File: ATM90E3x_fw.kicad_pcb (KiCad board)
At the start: 2 copper layers, 50.8 x 50.8 mm, 77 parts, among them IC1 ATM90E36_ATM90E36, J1 RJ45, J2 CONN_01X04, J3 GS3, J4 GS3, J5 GS3, J6 CONN_01X06, J7 CONN_01X06, J8 CONN_01X04, J9 GROVE-SMD-90D, U1 ROF-78E, Y1 Crystal_GND24

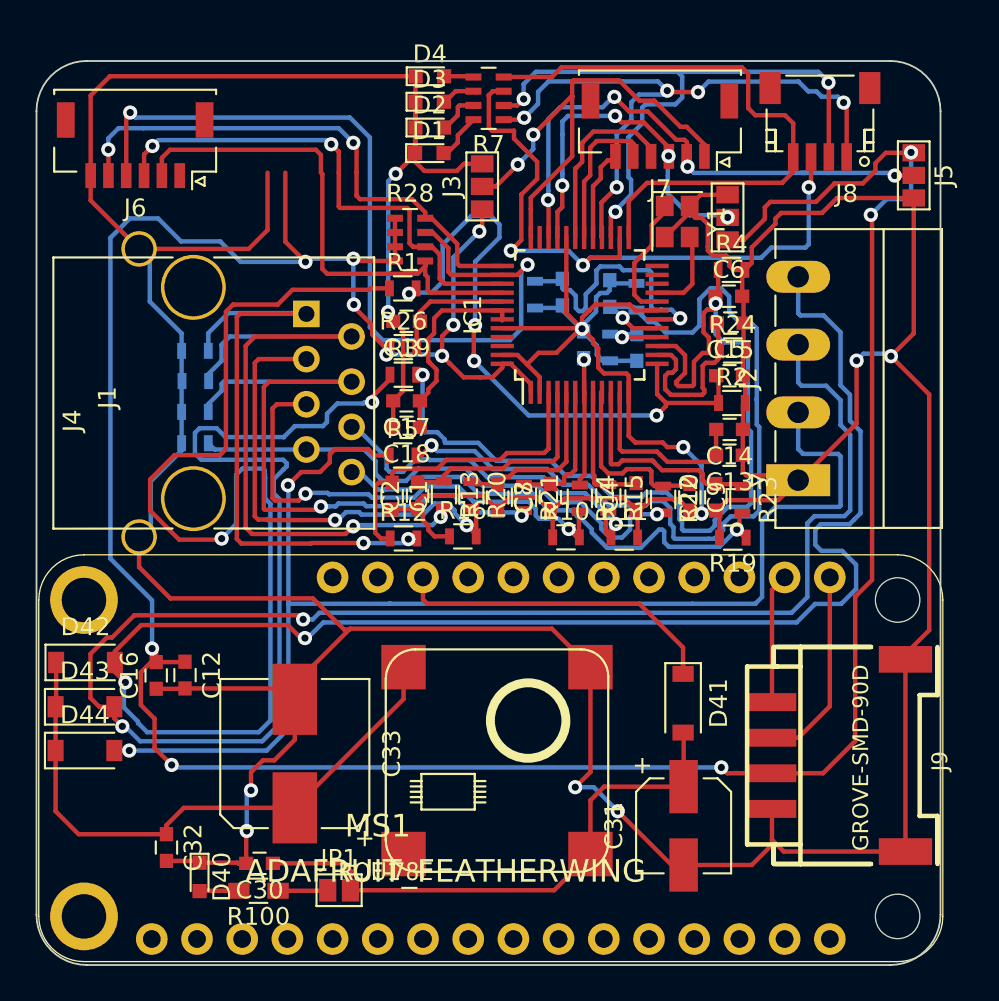
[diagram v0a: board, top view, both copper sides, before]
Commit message: Urbito delivery
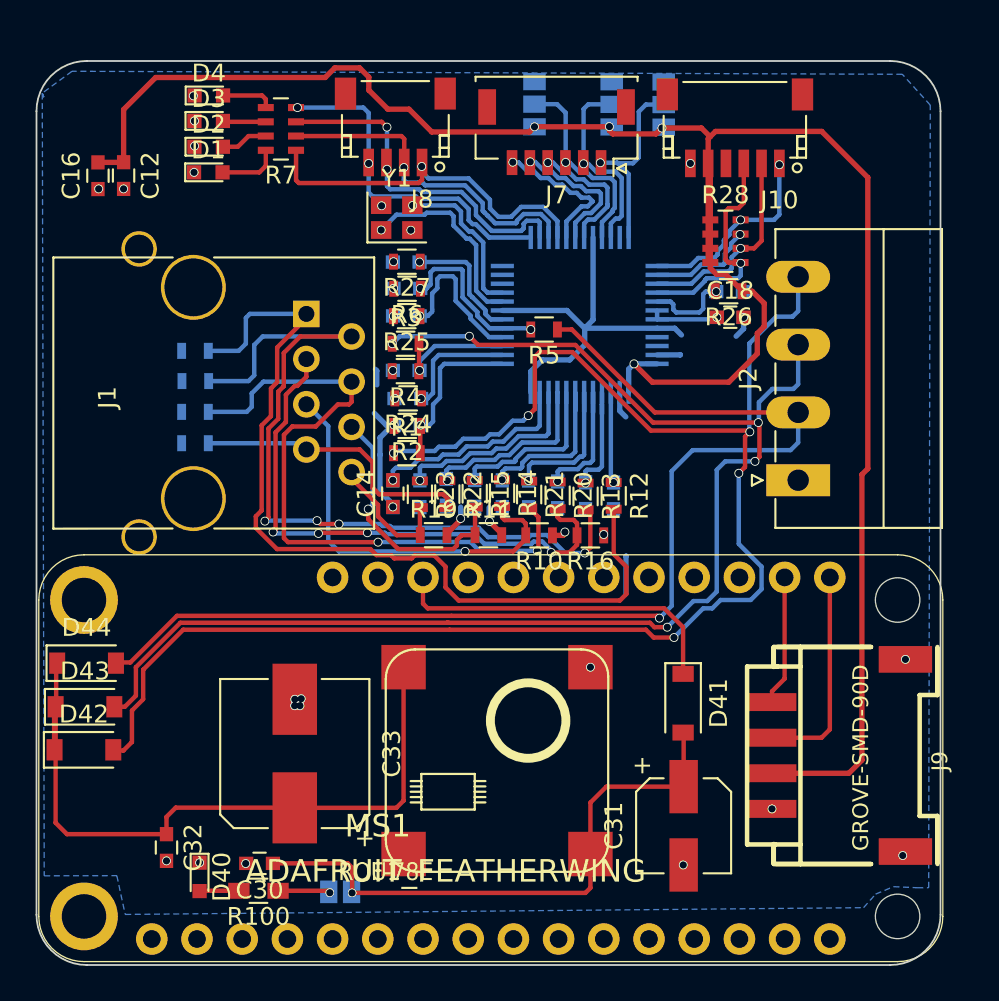
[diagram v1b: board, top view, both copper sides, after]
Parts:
- removed J6: CONN_01X06, Connectors_JST:JST_SHL_SM06B-SHLS-TF_06x1.00mm_Angled
- added J10: CONN_01X06, Connectors_JST:JST_SH_SM06B-SRSS-TB_06x1.00mm_Angled, F.Cu at (146.1, 44.7)
- added LOGO1: OPEN_HARDWARE_1, Symbols:OSHW-Logo2_7.3x6mm_SilkScreen, B.Cu at (135.6, 81.5)
- C1, C10, C13, C15, C17, C19, C2, C4, C5, C6, C7, C8, C9, IC1, J3, J4, J5, JP1: moved to B.Cu
- R25, R27, R6: moved to F.Cu
- moved C12 28.3 mm to (111.8, 47.3)
- moved C16 28.3 mm to (110.3, 47.3)
- moved J8 23.9 mm to (127.0, 44.6)
- moved C14 19.3 mm to (126.9, 65.2), turned to 90 degrees
- moved C18 19.2 mm to (145.8, 55.3), turned to 0 degrees
- moved R4 19.2 mm to (127.6, 58.3), turned to 180 degrees
- moved C13 19.0 mm to (126.9, 65.2), turned to 90 degrees
- moved C17 18.8 mm to (145.8, 55.3), turned to 0 degrees
- moved C15 18.6 mm to (127.7, 59.9), turned to 0 degrees
- moved C6 18.6 mm to (127.6, 58.3), turned to 180 degrees
- moved R26 18.5 mm to (145.8, 53.8), turned to 180 degrees
- moved R24 18.4 mm to (127.7, 59.8), turned to 180 degrees
- moved C5 18.3 mm to (127.7, 61.3), turned to 180 degrees
- moved R2 18.3 mm to (127.7, 61.4), turned to 180 degrees
- moved C19 18.2 mm to (145.8, 53.8), turned to 0 degrees
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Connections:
- MS1 pad 2: +3V3 -> Net-(MS1-Pad2)
- MS1 pad 4: GND -> Net-(MS1-Pad4)
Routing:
- net GND: track 345.9 -> 40.2 mm, vias 11 -> 33
- net +3V3: track 172.6 -> 123.0 mm, vias 12 -> 4
- net V2P: track 51.8 -> 7.03 mm, vias 2 -> 1
- net SCLK: track 48.9 -> 6.09 mm, vias 2 -> 1
- net UA: track 128.6 -> 88.5 mm, vias 3 -> 5
- net V3P: track 49.4 -> 9.87 mm
- net UB: track 109.9 -> 78.0 mm, vias 3 -> 5
- net V1P: track 36.5 -> 9.13 mm, vias 4 -> 1
- net IN_IN: track 28.1 -> 7.48 mm, vias 1 -> 0
- net PM1: track 30.5 -> 11.0 mm, vias 4 -> 1
- net CS: track 30.2 -> 11.3 mm
- net CF2: track 38.0 -> 20.1 mm, vias 3 -> 2
- net MISO: track 28.7 -> 11.6 mm, vias 2 -> 1
- net CF3: track 36.2 -> 19.2 mm, vias 3 -> 1
- net DMA: track 27.2 -> 11.0 mm, vias 2 -> 1
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- added copper zone on B.Cu, net GND
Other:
- net class +3v3 added: clearance 0.2, trace_width 0.3, via_dia 0.8, via_drill 0.4
- net class Default: clearance 0.2 -> 0.1; trace_width 0.25 -> 0.3; via_dia 0.8 -> 0.5
- net class GND added: clearance 0.2, trace_width 0.3, via_dia 0.8, via_drill 0.4
- net class VCC added: clearance 0.2, trace_width 0.3, via_dia 0.8, via_drill 0.4
- rule trace_clearance: 0.2 -> 0.1
